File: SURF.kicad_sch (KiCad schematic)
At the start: 40 parts, among them J1 Conn_01x21_Pin, J2 Conn_01x21_Pin, Q3 Q_Dual_PMOS_S1G1D2S2G2D1, SW1 SW_Omron_B3FS, SW2 SW_Omron_B3FS, U1 ESP32-S2-MINI-2, U10 COMM_10_RIGHT, U11 CONN_10_LEFT, U2 UART, U6 NCP164CSN300T1G, U7 XC6206PxxxMR, U8 XC6206PxxxMR

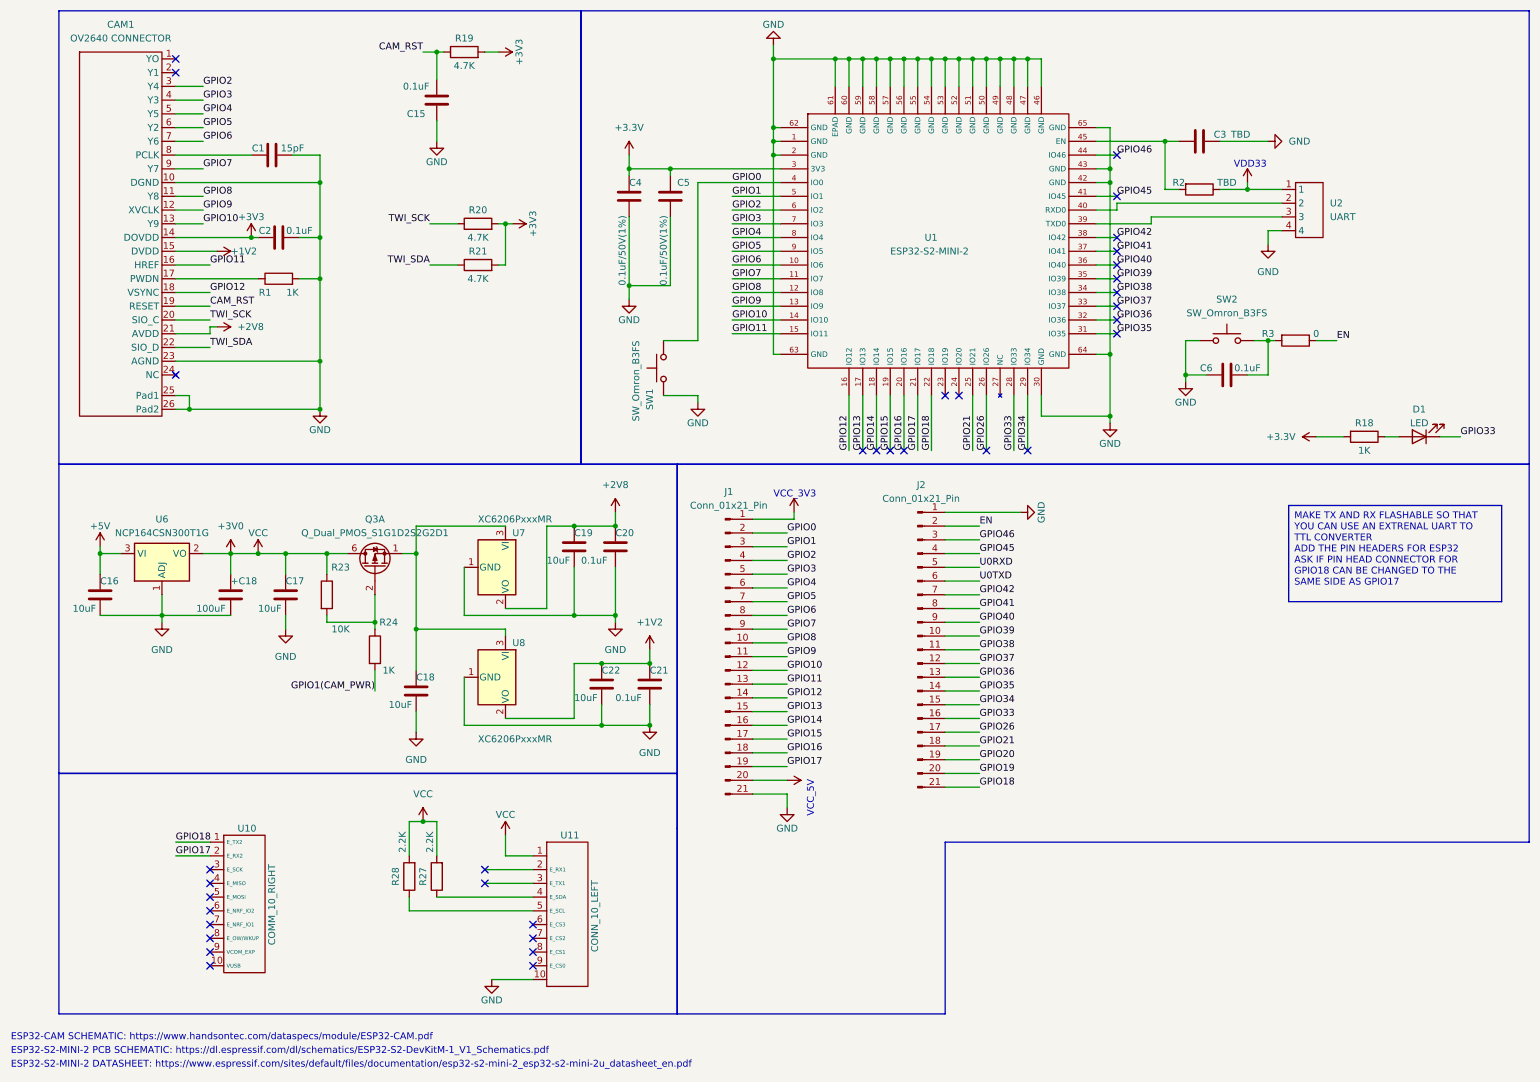
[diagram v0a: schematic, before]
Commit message: update
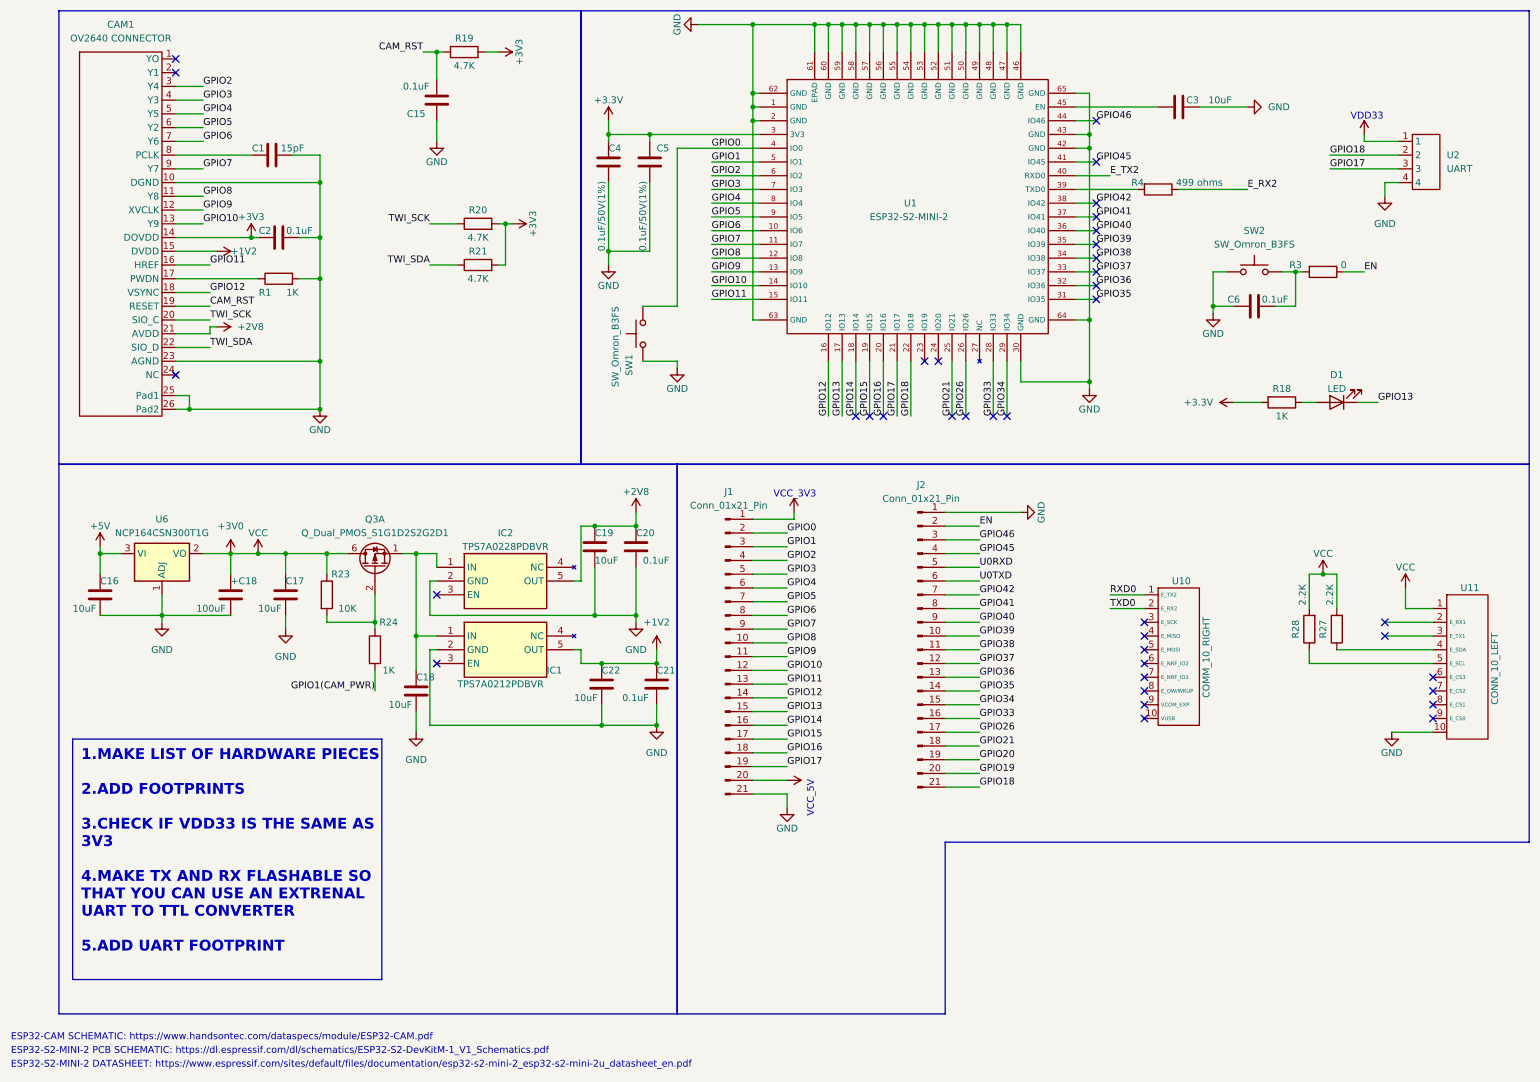
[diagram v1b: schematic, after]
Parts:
- removed R2: TBD, symbol Device:R
- removed U7, U8: XC6206PxxxMR, Package_TO_SOT_SMD:SOT-23-3, symbol Regulator_Linear:XC6206PxxxMR
- added IC1: TPS7A0212PDBVR, SOT95P280X145-5N, symbol TPS7A0212PDBVR:TPS7A0212PDBVR
- added IC2: TPS7A0228PDBVR, SOT95P280X145-5N, symbol TPS7A0228PDBVR:TPS7A0228PDBVR
- added R4: 499 ohms, symbol Device:R
- C3: value TBD -> 10uF
- SW1, SW2: footprint (none) -> B3FS:B3FS1012
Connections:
- net +1V2: now also IC1.5 (OUT)
- net +2V8: now also IC2.5 (OUT)
- net GND: now also IC1.2 (GND), IC2.2 (GND)
- net GPIO13: now also D1.1 (K)
- net GPIO17: now also U2.3; no longer U10.2 (E_RX2)
- net GPIO18: now also U2.2; no longer U10.1 (E_TX2)
- net GPIO33: no longer D1.1 (K)
- net at C18.1, Q3.1 (S): now also IC1.1 (IN), IC2.1 (IN)
- net E_TX2: now reaches U1.40 (RXD0)
- net E_TX2: no longer U2.2
- net at U1.39 (TXD0): now also R4.2; no longer U2.3
- new net E_RX2: R4.1
- new net RXD0: U10.1 (E_TX2)
- new net TXD0: U10.2 (E_RX2)
- no-connect marks 35 -> 38
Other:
- moved on the sheet: C19, C20, C21, C3, C4, C5, C6, D1, R18, R27, R28, R3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
